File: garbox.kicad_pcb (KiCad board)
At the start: 4 copper layers, 58.4 x 65.3 mm, 79 parts, among them J1 Batteries Terminal, J2 Speaker Terminals, J3 USB4056-03-A_REVA2, J4 MSD-4-A, U1 ESP32-S3-WROOM-1-N4R8, U10 FT231XQ-T, U2 CS4344-CZZR, U3 PAM8302AASCR, U4 AMS1117-3.3, U5 AMS1117-5.0, U6 BQ25887RGER, U7 CPDQ5V0-HF, U8 CPDQ5V0-HF, U9 CPDQ5V0-HF

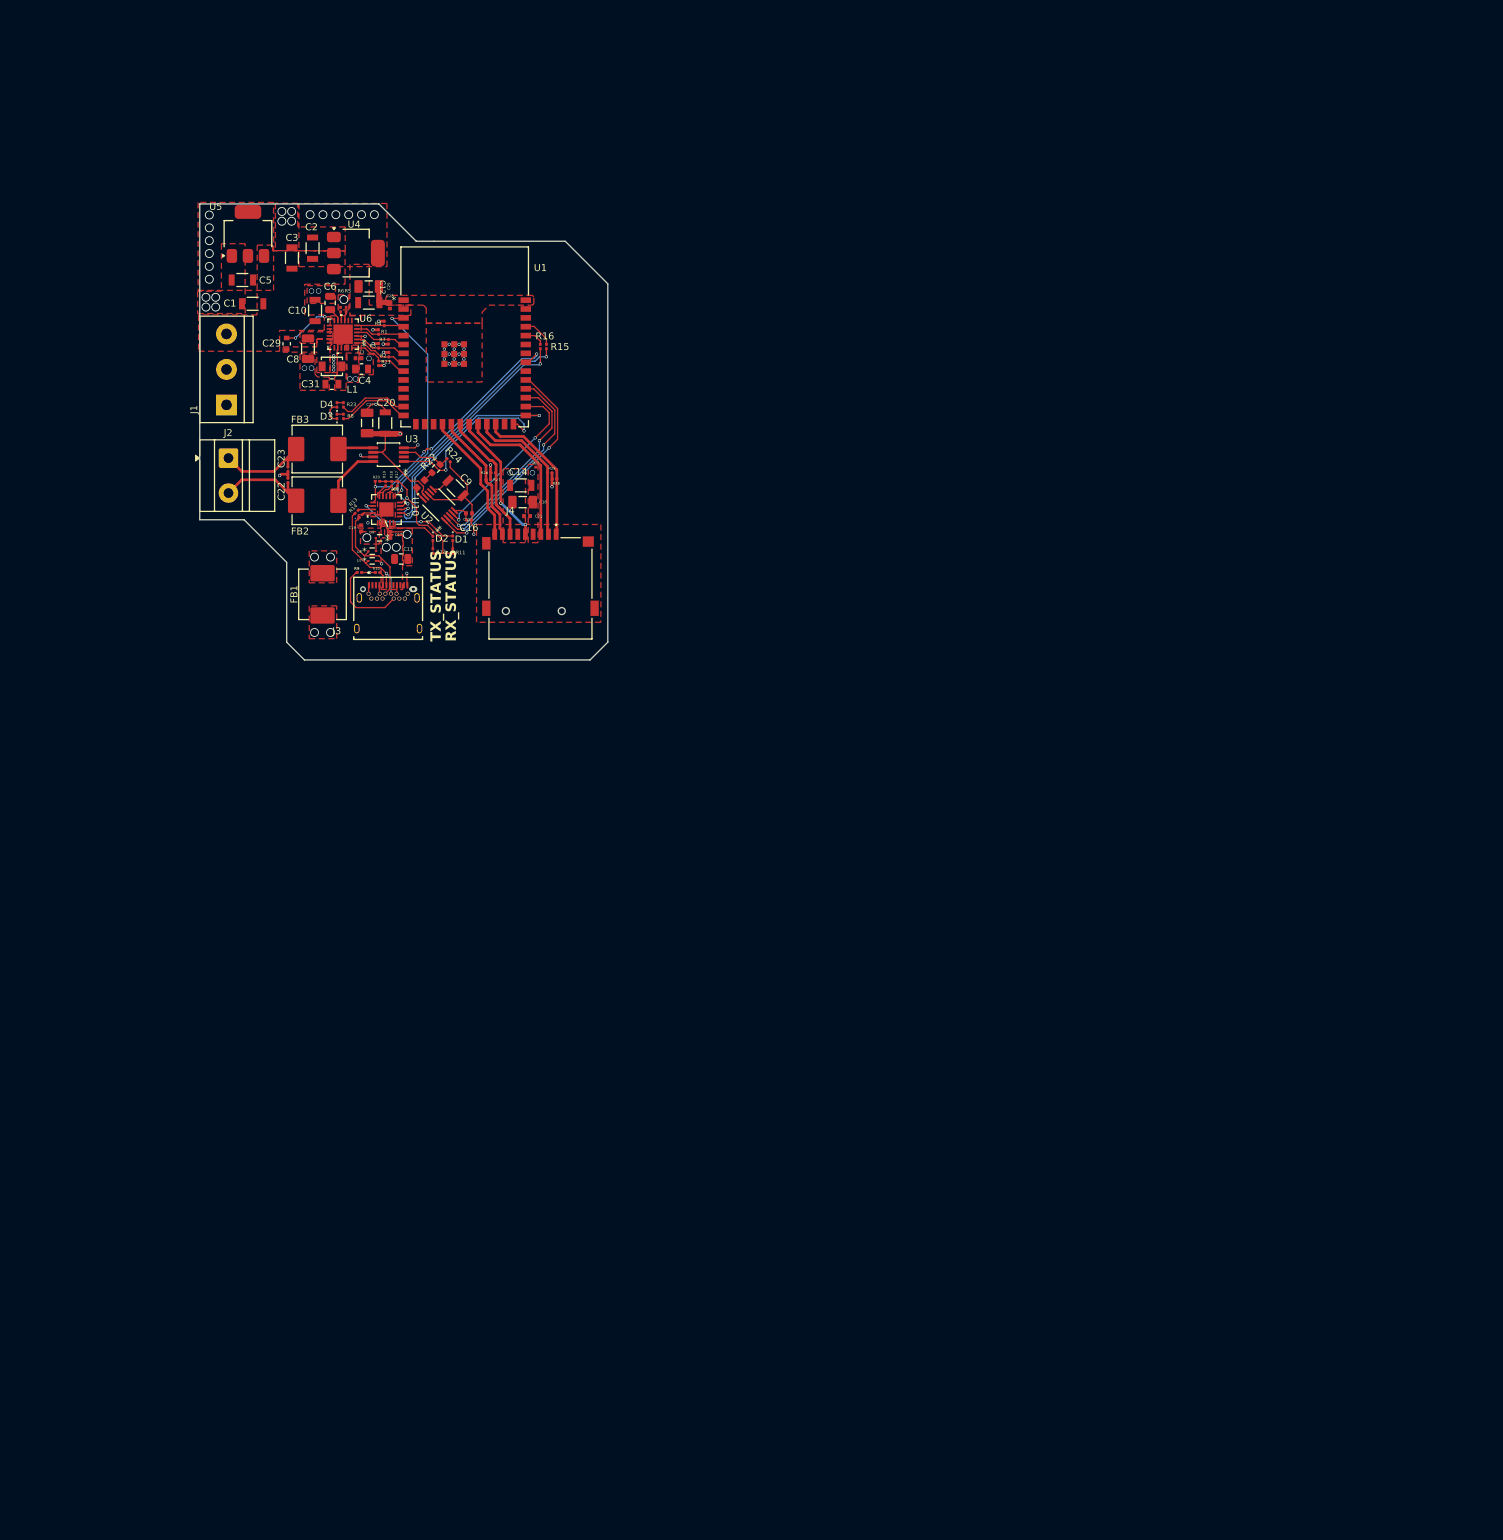
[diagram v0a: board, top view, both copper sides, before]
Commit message: meant to put these in the last commit
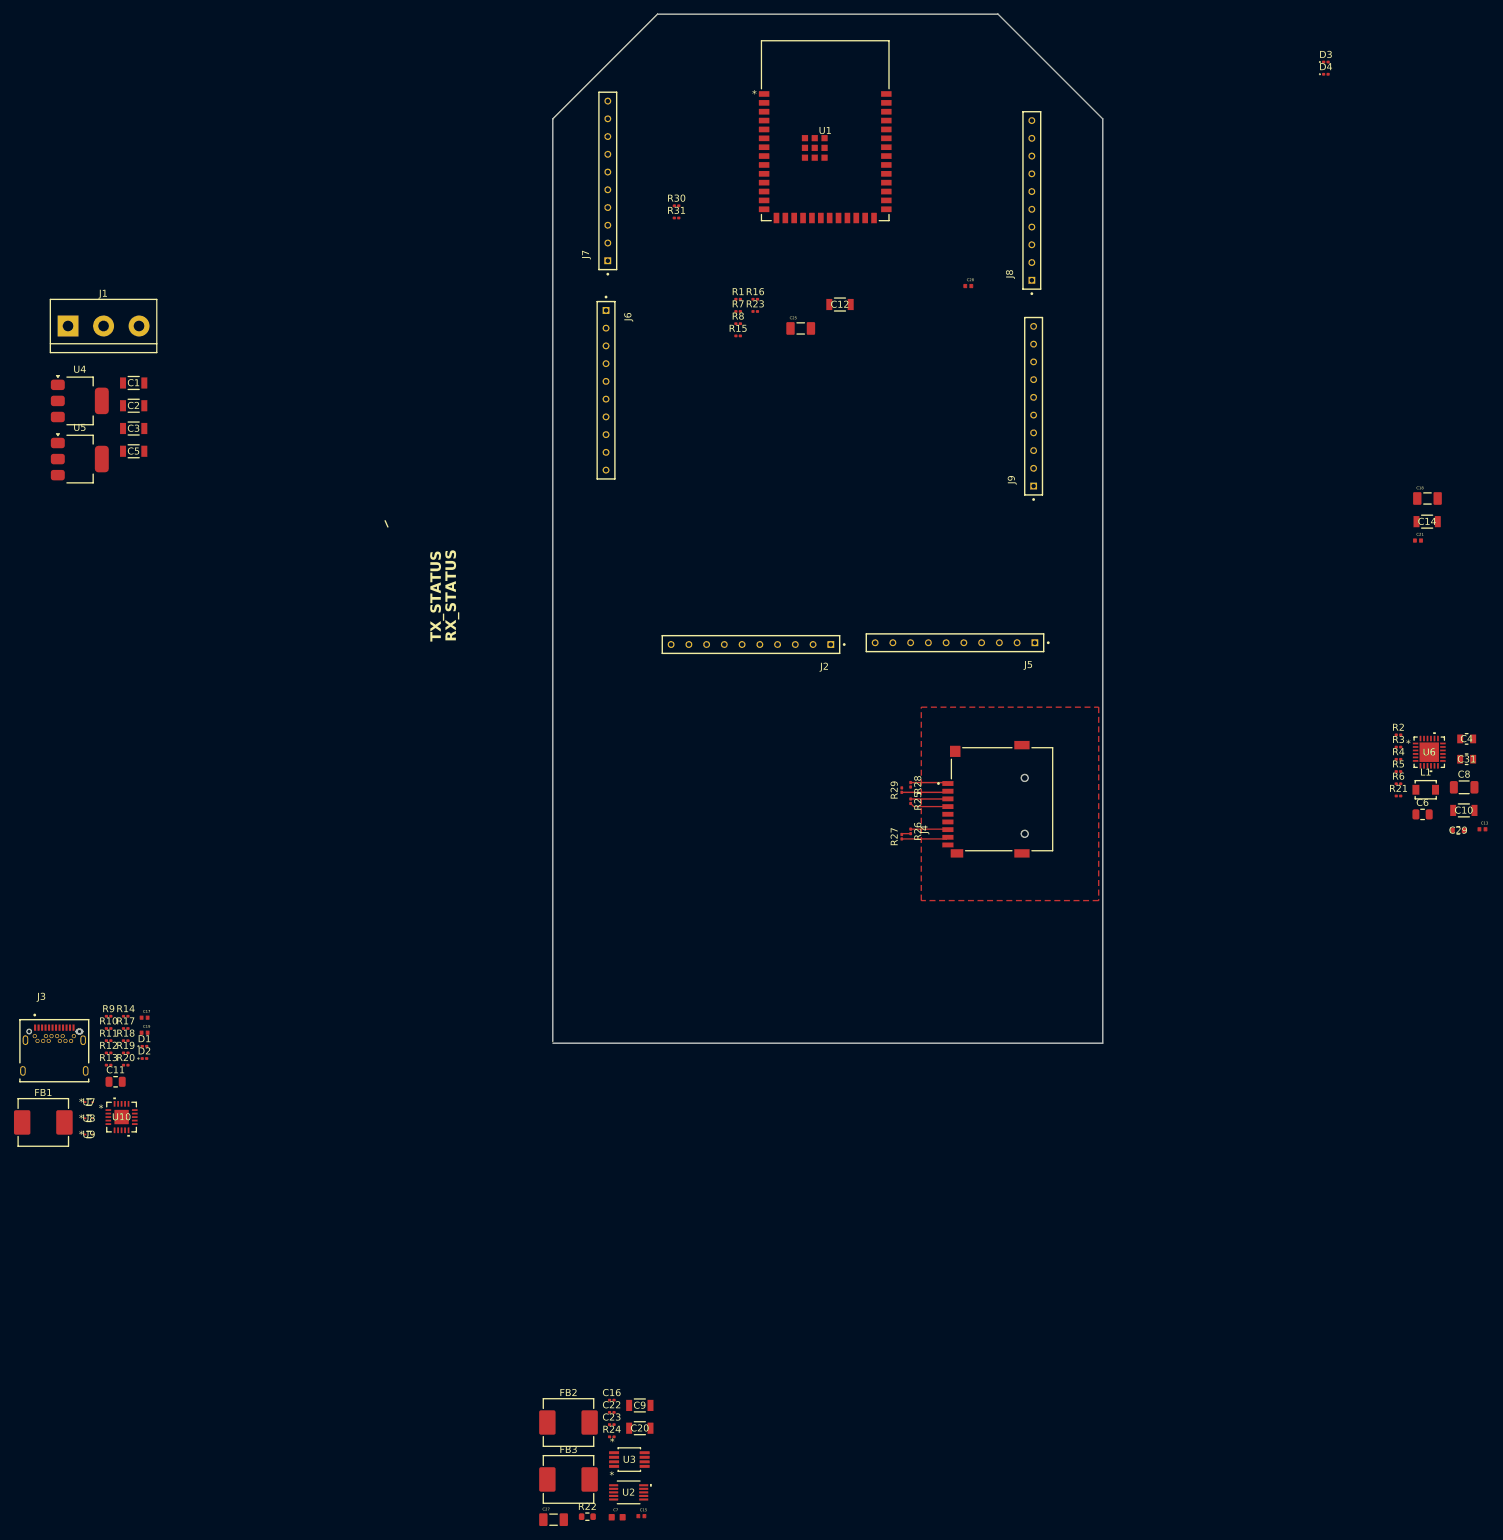
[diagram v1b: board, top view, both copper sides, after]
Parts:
- added J5: SD_Header, TS_110_G_A:SAMTEC_TS-110-G-A, F.Cu at (163.5, 111.3)
- added J6: PowerBreakoutHeader, TS_110_G_A:SAMTEC_TS-110-G-A, F.Cu at (113.5, 75.2)
- added J7: BMS_Header, TS_110_G_A:SAMTEC_TS-110-G-A, F.Cu at (113.8, 45.2)
- added J8: Audio_Header, TS_110_G_A:SAMTEC_TS-110-G-A, F.Cu at (174.5, 48.0)
- added J9: GPIO_Header, TS_110_G_A:SAMTEC_TS-110-G-A, F.Cu at (174.8, 77.5)
- added R30: 22, Resistor_SMD:R_0201_0603Metric, F.Cu at (123.6, 48.8)
- added R31: 22, Resistor_SMD:R_0201_0603Metric, F.Cu at (123.6, 50.5)
- J2: value Speaker Terminals -> USB_Header; footprint TerminalBlock_MetzConnect:TerminalBlock_MetzConnect_Type011_RT05502HBLC_1x02_P5.00mm_Horizontal -> TS_110_G_A:SAMTEC_TS-110-G-A
- moved C29 181.6 mm to (235.6, 138.2), turned to 0 degrees
- moved C10 179.4 mm to (236.4, 135.3), turned to 0 degrees
- moved C8 177.0 mm to (236.4, 132.0), turned to 0 degrees
- moved C13 174.5 mm to (239.0, 138.0)
- moved C6 172.7 mm to (230.4, 135.9), turned to 0 degrees
- moved C31 171.1 mm to (236.8, 128.0)
- moved L1 167.9 mm to (230.9, 132.4)
- moved C4 166.8 mm to (236.8, 125.1)
- moved U6 166.6 mm to (231.4, 127.0), turned to 0 degrees
- moved R6 166.0 mm to (227.0, 131.5), turned to 0 degrees
- moved R5 164.5 mm to (227.0, 129.8), turned to 0 degrees
- moved C27 159.3 mm to (106.0, 236.9), turned to 0 degrees
- moved R21 158.6 mm to (227.0, 133.3), turned to 0 degrees
- moved R4 158.0 mm to (227.0, 128.0), turned to 0 degrees
- moved R3 156.9 mm to (227.0, 126.3), turned to 0 degrees
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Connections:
- net /Audio/AMP_ENABLE renamed /AMP_ENABLE
- net /Audio/i2s_LRCK renamed /i2s_LRCK
- net /Audio/i2s_MCLK renamed /i2s_MCLK
- net /Audio/i2s_SCLK renamed /i2s_SCLK
- net /Audio/i2s_SDIN renamed /i2s_SDIN
- net /BatteryManagement/BMS_Interrupt renamed /BMS_Interrupt
- net /BatteryManagement/ChargeStatus renamed /ChargeStatus
- net /BatteryManagement/PSEL renamed /PSEL
- net /BatteryManagement/PowerGood renamed /PowerGood
- net /BatteryManagement/SCL renamed /SCL
- net /BatteryManagement/SDA renamed /SDA
- C11 pad 2: /BatteryManagement/PowerIn -> /USB_PowerSupply
- C13 pad 1: /BatteryManagement/PowerIn -> /USB_PowerSupply
- C17 pad 2: /BatteryManagement/PowerIn -> /USB_PowerSupply
- C2 pad 2: +3.3V -> /PowerRegulation/3V3
- C22 pad 1: /Audio/Spk- -> /Spk-
- C23 pad 1: /Audio/Spk+ -> /Spk+
- C4 pad 1: /BatteryManagement/PowerIn -> /USB_PowerSupply
- C5 pad 2: +5V -> /PowerRegulation/5V
- FB2 pad 1: /Audio/Spk- -> /Spk-
- FB3 pad 1: /Audio/Spk+ -> /Spk+
- J3 pad A4: /BatteryManagement/PowerIn -> /USB_PowerSupply
- J3 pad A9: /BatteryManagement/PowerIn -> /USB_PowerSupply
- J3 pad B4: /BatteryManagement/PowerIn -> /USB_PowerSupply
- J3 pad B9: /BatteryManagement/PowerIn -> /USB_PowerSupply
- R15 pad 1: /USB_Data&Power/FLASH_RXD -> /FLASH_RXD
- R16 pad 1: /USB_Data&Power/FLASH_TXD -> /FLASH_TXD
- R20 pad 2: /USB_Data&Power/CTS# -> /CTS#
- R23 pad 1: Net-(U1-IO19) -> /GPLED_01
- R8 pad 1: Net-(U1-IO20) -> /GPLED_02
- U1 pad 10: unconnected-(U1-IO17-Pad10) -> /GPLED_01
- U1 pad 11: unconnected-(U1-IO18-Pad11) -> /GPLED_02
- U1 pad 12: unconnected-(U1-IO8-Pad12) -> /GPIO_08
- U1 pad 15: unconnected-(U1-IO3-Pad15) -> /GPIO_03
- U1 pad 16: unconnected-(U1-IO46-Pad16) -> /GPIO_46
- U1 pad 17: unconnected-(U1-IO9-Pad17) -> /GPIO_09
- U1 pad 25: unconnected-(U1-IO48-Pad25) -> /GPIO_48
- U1 pad 27: /USB_Data&Power/DTR# -> /FLASH_TXD
- U1 pad 3: /USB_Data&Power/RTS# -> /RTS#
- U1 pad 32: unconnected-(U1-IO39-Pad32) -> /GPIO_39
- U1 pad 33: /USB_Data&Power/CTS# -> /DTR#
- U1 pad 34: unconnected-(U1-IO41-Pad34) -> /GPIO_41
- U1 pad 35: unconnected-(U1-IO42-Pad35) -> /GPIO_42
- U1 pad 38: unconnected-(U1-IO2-Pad38) -> /GPIO_02
- U1 pad 39: unconnected-(U1-IO1-Pad39) -> /GPIO_01
- U10 pad 1: /USB_Data&Power/FLASH_RXD -> /FLASH_RXD
- U10 pad 12: /BatteryManagement/PowerIn -> /USB_PowerSupply
- U10 pad 17: /USB_Data&Power/FLASH_TXD -> /FLASH_TXD
- U10 pad 18: /USB_Data&Power/DTR# -> /DTR#
- U10 pad 19: /USB_Data&Power/RTS# -> /RTS#
- U10 pad 6: /USB_Data&Power/CTS# -> /CTS#
- U4 pad 2: +3.3V -> /PowerRegulation/3V3
- U5 pad 2: +5V -> /PowerRegulation/5V
- U6 pad 23: /BatteryManagement/PowerIn -> /USB_PowerSupply
- U9 pad 1: /BatteryManagement/PowerIn -> /USB_PowerSupply
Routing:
- net +5V: track 82.5 -> 0.00 mm, vias 7 -> 0
- net GND: track 49.0 -> 0.00 mm, vias 45 -> 0
- net /USB_Data&Power/CTS#: track 36.4 -> 0.00 mm, vias 4 -> 0
- net /BatteryManagement/PowerIn: track 34.3 -> 0.00 mm, vias 4 -> 0
- net /USB_Data&Power/FLASH_TXD: track 34.2 -> 0.00 mm, vias 2 -> 0
- net /USB_Data&Power/RTS#: track 34.0 -> 0.00 mm, vias 2 -> 0
- net /i2s_SDIN: track 33.4 -> 0.00 mm, vias 2 -> 0
- net /USB_Data&Power/DTR#: track 33.3 -> 0.00 mm, vias 2 -> 0
- net /USB_Data&Power/FLASH_RXD: track 31.9 -> 0.00 mm, vias 2 -> 0
- net /i2s_SCLK: track 31.0 -> 0.00 mm, vias 2 -> 0
- net /i2s_LRCK: track 28.8 -> 0.00 mm, vias 2 -> 0
- net Net-(U10-3V3OUT): track 27.6 -> 0.00 mm, vias 2 -> 0
- net /i2s_MCLK: track 25.9 -> 0.00 mm, vias 2 -> 0
- net /AMP_ENABLE: track 25.7 -> 0.00 mm, vias 2 -> 0
- net /BatteryManagement/PackMid: track 20.9 -> 0.00 mm, vias 1 -> 0
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- removed copper zone on F.Cu, net +3.3V
- removed copper zone on In2.Cu, net +3.3V
- removed copper zone on F.Cu, net +5V
- removed copper zone on F.Cu, net /BatteryManagement/PackMid
- removed copper zone on F.Cu, net /BatteryManagement/PackPlus
- removed copper zone on F.Cu, net /BatteryManagement/PowerIn
- removed copper zone on In2.Cu, net /BatteryManagement/PowerIn
- removed copper zone on In1.Cu, net GND
- removed copper zone on F.Cu, net Net-(C29-Pad1)
- removed copper zone on F.Cu, net Net-(C31-Pad2)
- removed copper zone on F.Cu, net Net-(C8-Pad1)
- removed copper zone on F.Cu, net Net-(J3-SHELL_GND)
- removed copper zone on In1.Cu, net Net-(J3-SHELL_GND)
- removed copper zone on F.Cu, net Net-(U10-3V3OUT)
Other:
- board size 58.4 x 65.3 mm -> 78.7 x 147.3 mm
